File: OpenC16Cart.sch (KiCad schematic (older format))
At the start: 15 parts, among them J1 CONN_02X03, J11 CONN_01X03, J12 CONN_01X03, J2 CONN_01X03, J21 CONN_01X03, J22 CONN_01X03, J3 CONN_01X03, J4 CONN_02X03, J5 CONN_01X03, J6 CONN_01X03, J7 C16-Exp-Port, U1 27512 - LO ROM, U2 27512 - HI ROM

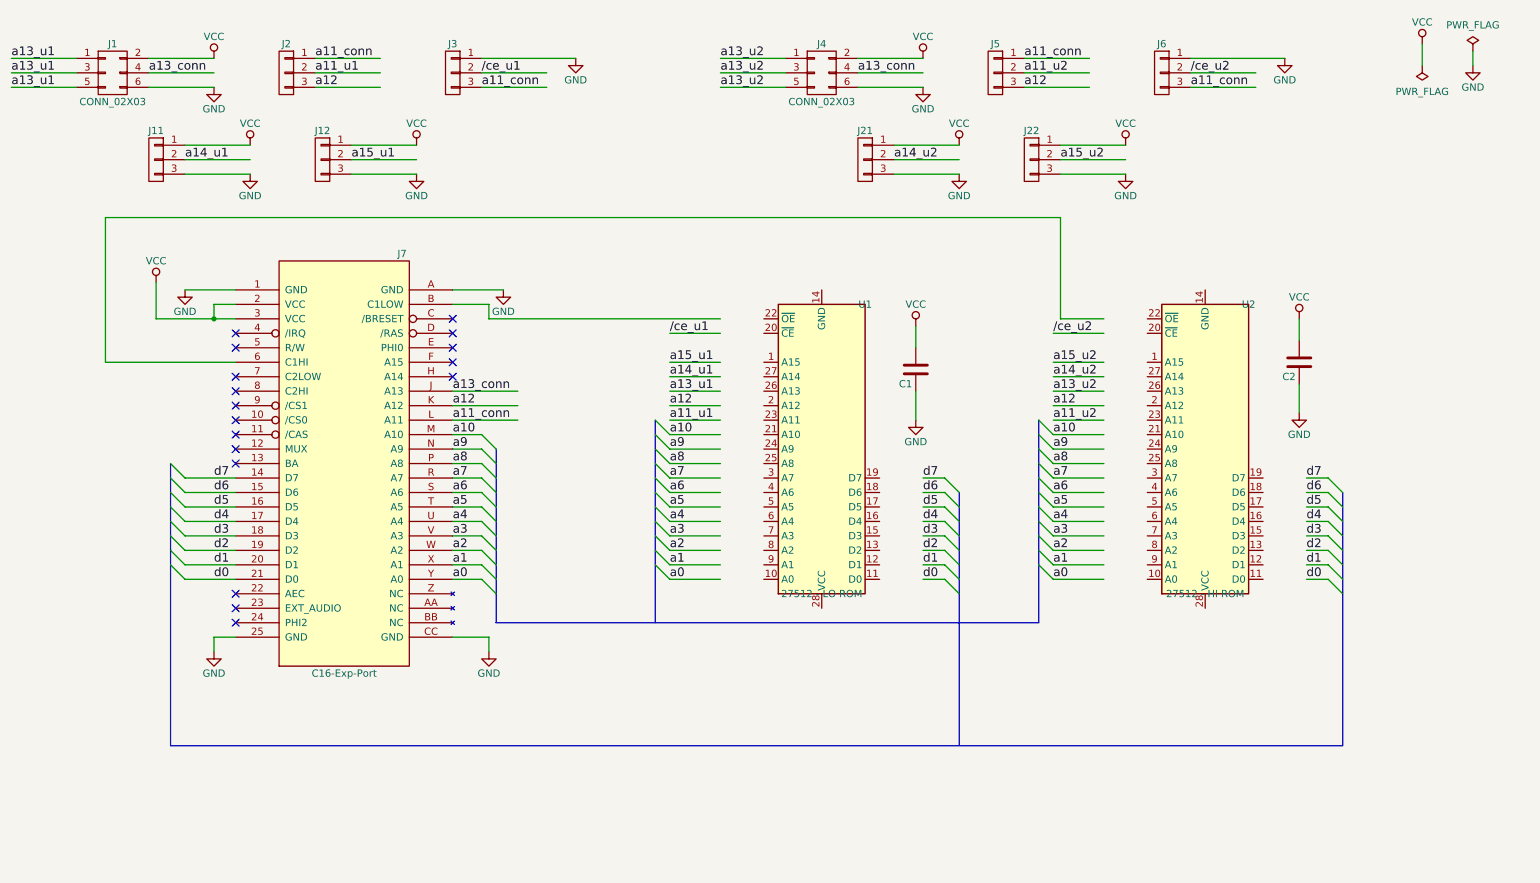
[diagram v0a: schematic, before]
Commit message: Much better
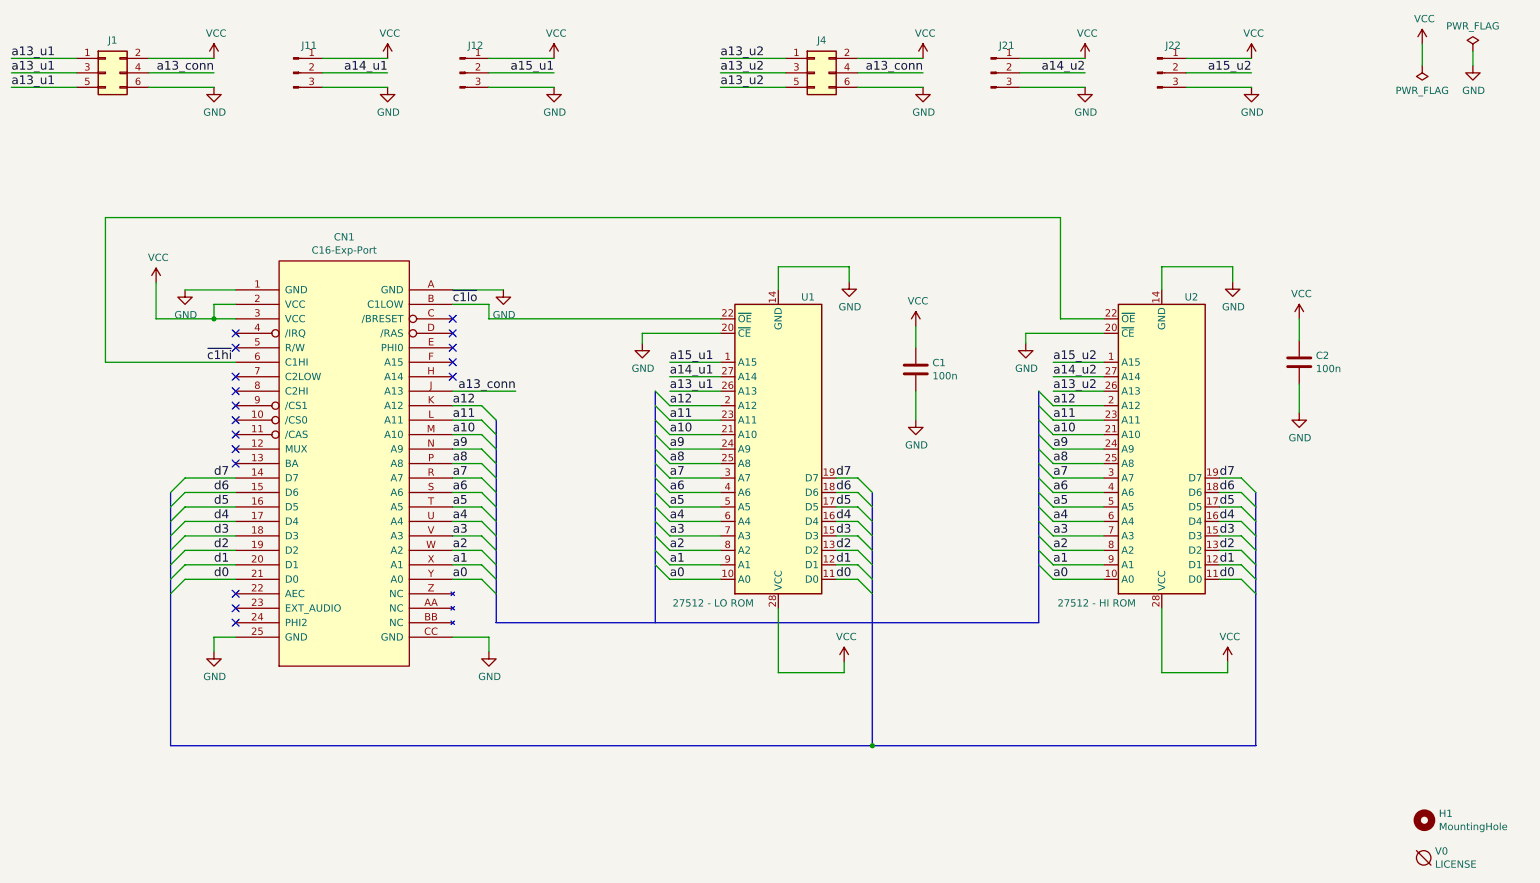
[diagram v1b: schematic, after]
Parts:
- removed C1, C2: C, Capacitors_SMD:C_0805_HandSoldering, symbol C
- removed J1, J4: CONN_02X03, OpenC16Cart:Pin_Header_Straight_2x03-ModSilkS, symbol CONN_02X03
- removed J11, J12, J2, J21, J22, J3, J5, J6: CONN_01X03, OpenC16Cart:Pin_Header_Straight_1x03-ModSilkS, symbol CONN_01X03
- removed J7: C16-Exp-Port, OpenC16Cart:C16_Cart_Conn, symbol C16-Exp-Port
- removed U1: 27512 - LO ROM, OpenC16Cart:dil_28-600_socket_ThinSilkS, symbol 27512
- removed U2: 27512 - HI ROM, OpenC16Cart:dil_28-600_socket_ThinSilkS, symbol 27512
- added C1, C2: 100n, Capacitor_THT:C_Disc_D7.0mm_W2.5mm_P5.00mm, symbol Device:C
- added CN1: C16-Exp-Port, OpenC16Cart:C16_Cart_Conn, symbol C16-Exp-Port:C16-Exp-Port
- added H1: MountingHole, MountingHole:MountingHole_3.2mm_M3, symbol Mechanical:MountingHole
- added J1, J4: Conn_02x03_Odd_Even, Connector_PinHeader_2.54mm:PinHeader_2x03_P2.54mm_Vertical, symbol Connector_Generic:Conn_02x03_Odd_Even
- added J11, J12, J21, J22: Conn_01x03_Male, Connector_PinHeader_2.54mm:PinHeader_1x03_P2.54mm_Vertical, symbol Connector:Conn_01x03_Male
- added U1: 27512 - LO ROM, Package_DIP:DIP-28_W15.24mm_Socket_LongPads, symbol Memory_EPROM:27C512
- added U2: 27512 - HI ROM, Package_DIP:DIP-28_W15.24mm_Socket_LongPads, symbol Memory_EPROM:27C512
- added V0: LICENSE, OpenC16Cart:cc_by_nc_sa, symbol void:Void
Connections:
- net labels added: a11, ~c1hi, ~c1lo
- net labels removed: /ce_u1, /ce_u2, a11_conn, a11_u1, a11_u2
- wire segments 132 -> 135
